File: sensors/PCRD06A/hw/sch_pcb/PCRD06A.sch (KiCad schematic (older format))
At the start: 37 parts, among them J1 3.6V, J11 HEADER_2x01_PARALLEL, J2 HEADER_2x01_PARALLEL, J3 HEADER_2x01_PARALLEL, J4 HEADER_2x01_PARALLEL, J5 HEADER_2x01_PARALLEL, J6 HEADER_2x01_PARALLEL, J7 HEADER_2x01_PARALLEL, M1 HOLE, M2 HOLE, M3 HOLE, M4 HOLE, M5 BMIS-209-C, M6 BMI-S-210-F, U2 AD8691, U4 TS7211, U5 TS5A4594

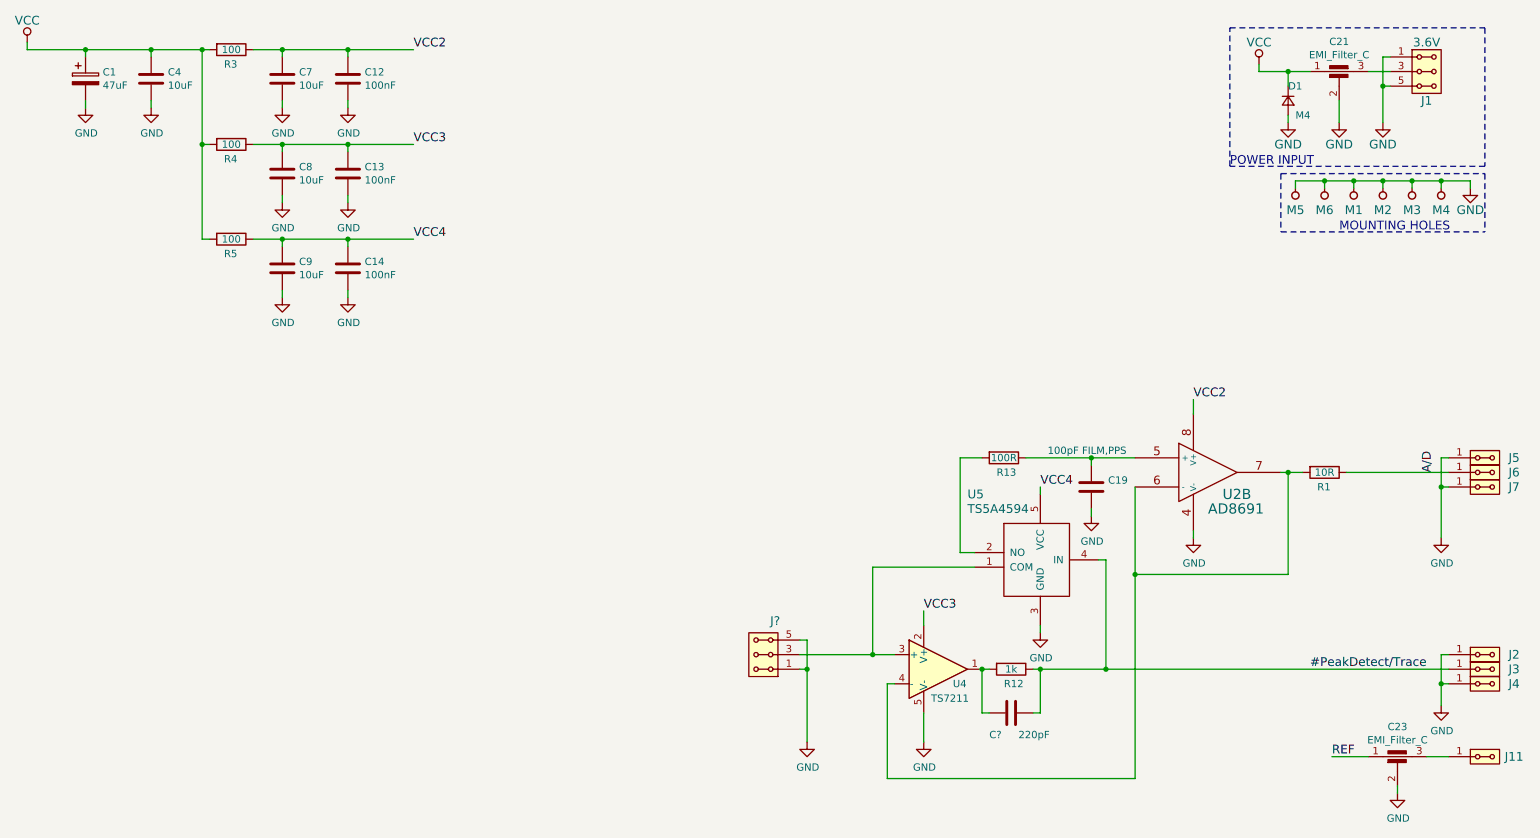
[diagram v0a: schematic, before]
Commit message: Edit
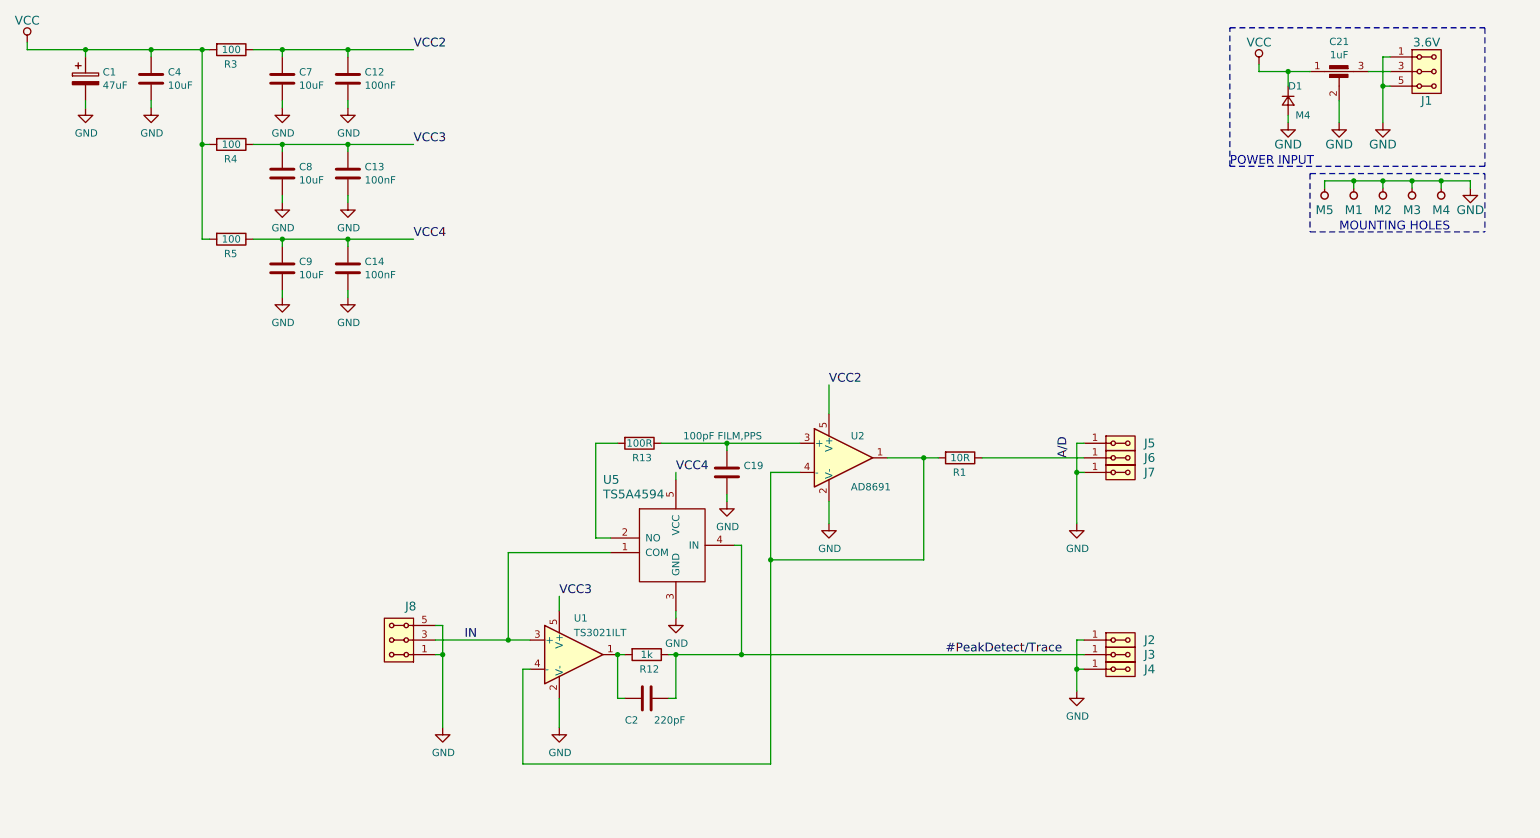
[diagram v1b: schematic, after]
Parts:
- removed C23: EMI_Filter_C, Mlab_L:FIR1, symbol Device:EMI_Filter_C
- removed J11: HEADER_2x01_PARALLEL, Mlab_Pin_Headers:Straight_2x01, symbol MLAB_HEADER:HEADER_2x01_PARALLEL
- removed M6: BMI-S-210-F, Mlab_Mechanical:BMI-S-210-F, symbol MLAB_MECHANICAL:HOLE
- removed U2: AD8691, Mlab_IO:SOIC-8_3.9x4.9mm_Pitch1.27mm, symbol MLAB_IO:AD8692
- removed U4: TS7211, Package_TO_SOT_SMD:SOT-23-5_HandSoldering, symbol Amplifier_Operational:OP179GRT
- added U1: TS3021ILT, Package_TO_SOT_SMD:SOT-23-5_HandSoldering, symbol MLAB_IO:AD8691
- added U2: AD8691, Package_TO_SOT_SMD:TSOT-23-5_HandSoldering, symbol MLAB_IO:AD8691
- C1: UST_ID (none) -> 5c70984412875079b91f8867
- C12, C13, C14: UST_ID (none) -> 5c70984712875079b91f8b4c
- C19: UST_ID (none) -> 5d47bf10128750448e6b4652
- C2: renamed from C?; UST_ID (none) -> 5c70984712875079b91f8b3f
- C21: value EMI_Filter_C -> 1uF; footprint Mlab_L:FIR1 -> Mlab_L:FIR_0805; UST_ID (none) -> 5c70984412875079b91f880f
- C4, C7, C8, C9: UST_ID (none) -> 5c70984812875079b91f8bbe
- D1: UST_ID (none) -> 5c70984512875079b91f88ac
- J8: renamed from J?; footprint (none) -> Mlab_Pin_Headers:Straight_2x03
- M5: value BMIS-209-C -> HOLE; footprint Mlab_Mechanical:BMIS-209-C -> RF_Shielding:Laird_Technologies_BMI-S-204-F_32.00x32.00mm
- R1: UST_ID (none) -> 5c70984512875079b91f896d
- R12: UST_ID (none) -> 5c70984512875079b91f898c
- R13, R3, R4, R5: UST_ID (none) -> 5c70984512875079b91f8977
- U5: UST_ID (none) -> 5c70984612875079b91f8a0d
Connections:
- net GND: now also U1.2 (V-), U2.2 (V-)
- net VCC2: now also U2.5 (V+)
- net VCC3: now also U1.5 (V+)
- net at C19.1, R13.1: now also U2.3 (+)
- net at R1.2: now also U1.4 (-), U2.1, U2.4 (-)
- net at C2.2, R12.2: now also U1.1
- net IN: now reaches J8.3, J8.4, U5.1 (COM)
- net IN: now also U1.3 (+)
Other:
- moved on the sheet: C19, C2, J2, J3, J4, J5, J6, J7, J8, R1, R12, R13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
